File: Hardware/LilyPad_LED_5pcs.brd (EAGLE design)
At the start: 27.4 x 12.8 mm, 26 parts

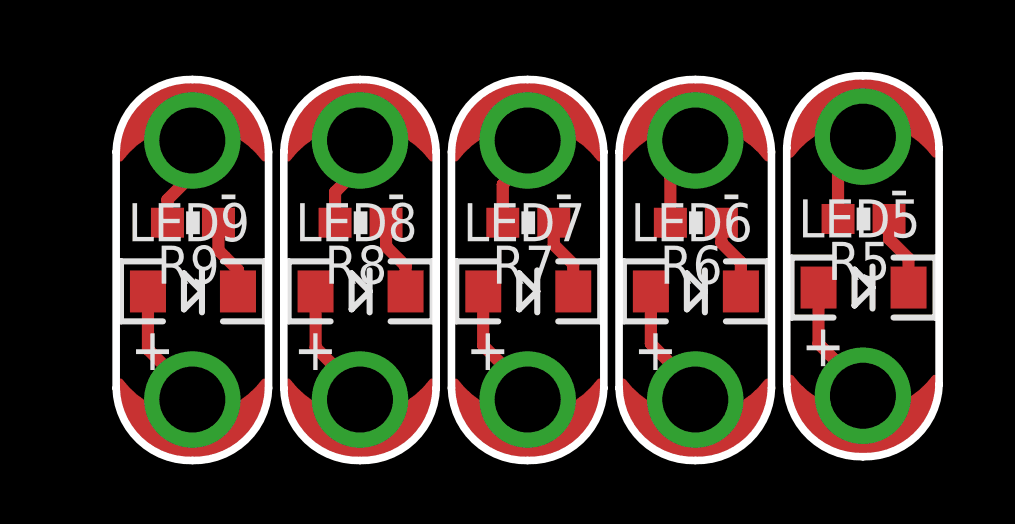
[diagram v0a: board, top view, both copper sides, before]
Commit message: updated brd and sch files
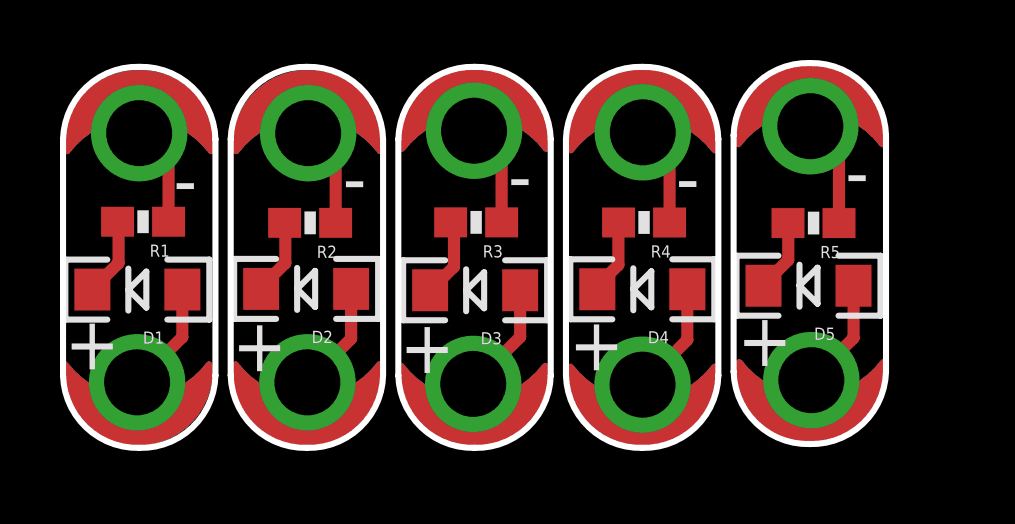
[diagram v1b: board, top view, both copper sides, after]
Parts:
- removed E$1: (no value), SparkFun-Aesthetics:CREATIVE_COMMONS
- removed LED+6, LED+7, LED+8, LED+9, LED-6, LED-7, LED-8, LED-9: SEWTAP6, LilyPad-Wearables:PETAL-SMALL
- removed LED5, LED6, LED7, LED8, LED9: White, SparkFun-LED:LED-1206
- removed LOGO10, LOGO6, LOGO7, LOGO8, LOGO9: LOGO-LPL, LilyPad-Wearables:LOGO-L
- removed R6, R7, R8, R9: 150, SparkFun:0603-RES
- added D1, D2, D3, D4, D5: WHITE, SparkFun-LED:LED-1206
- added FRAME1: FRAME-LETTER, SparkFun-Aesthetics:CREATIVE_COMMONS
- added LED+1, LED+2, LED+3, LED+4, LED-1, LED-2, LED-3, LED-4: SEWTAP6, LilyPad-Wearables:PETAL-SMALL-2SIDE
- added R1, R2, R3, R4: 150, SparkFun-Resistors:0603-RES
- added U$1, U$2, U$3, U$4, U$5: (no value), LilyPad-Wearables:LOGO-L
- added U$6: REVISION, SparkFun-Aesthetics:REVISION
- LED+5, LED-5: device LilyPad-Wearables:PETAL-SMALL -> LilyPad-Wearables:PETAL-SMALL-2SIDE
- R5: device SparkFun:0603-RES -> SparkFun-Resistors:0603-RES
- moved LED+5 1.80 mm to (25.1, 2.55)
- moved LED-5 1.79 mm to (25.0, 11.0)
- moved R5 1.67 mm to (25.2, 7.79)
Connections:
- removed net +5: LED+5.1, LED5.A
- removed net +6: LED+6.1, LED6.A
- removed net +7: LED+7.1, LED7.A
- removed net +8: LED+8.1, LED8.A
- removed net +9: LED+9.1, LED9.A
- removed net -5: LED-5.1, R5.2
- removed net -6: LED-6.1, R6.2
- removed net -7: LED-7.1, R7.2
- removed net -8: LED-8.1, R8.2
- removed net -9: LED-9.1, R9.2
- removed net N$10: LED9.C, R9.1
- removed net N$6: LED5.C, R5.1
- removed net N$7: LED6.C, R6.1
- removed net N$8: LED7.C, R7.1
- removed net N$9: LED8.C, R8.1
- new net 1: D1.A, LED+1.1
- new net 10: D4.A, LED+4.1
- new net 11: D4.C, R4.2
- new net 12: LED-4.1, R4.1
- new net 13: D5.A, LED+5.1
- new net 14: D5.C, R5.2
- new net 15: LED-5.1, R5.1
- new net 2: D1.C, R1.2
- new net 3: LED-1.1, R1.1
- new net 4: D2.A, LED+2.1
- new net 5: D2.C, R2.2
- new net 6: LED-2.1, R2.1
- new net 7: D3.A, LED+3.1
- new net 8: D3.C, R3.2
- new net 9: LED-3.1, R3.1
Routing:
- net +9: track 4.22 -> 0.00 mm
- net +7: track 4.22 -> 0.00 mm
- net +6: track 4.22 -> 0.00 mm
- net +5: track 4.22 -> 0.00 mm
- net +8: track 4.22 -> 0.00 mm
- net 10: track 0.00 -> 3.80 mm
- net 7: track 0.00 -> 3.77 mm
- net 13: track 0.00 -> 3.73 mm
- net 4: track 0.00 -> 3.72 mm
- net 1: track 0.00 -> 3.72 mm
- net 15: track 0.00 -> 3.62 mm
- net 9: track 0.00 -> 3.44 mm
- net 12: track 0.00 -> 3.37 mm
- net 6: track 0.00 -> 3.37 mm
- net 3: track 0.00 -> 3.36 mm
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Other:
- outline, holes or cut-outs redrawn
- board text added: "L. Buechley"
- board text added: "M. West"
- board text removed: "All Units Inches"
- board text removed: "Board Thickness: 0.032" Puprle Silk"
- board text removed: "Mary West"
- board text removed: "V Scoring (0.02" between parts)"
- board text removed: "White"
- board text removed: "white"
